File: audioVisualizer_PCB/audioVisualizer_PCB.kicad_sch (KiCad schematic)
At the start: 33 parts, among them J1 USB_C_Receptacle_USB2.0_16P, J3 SPI_LED_MATRIX, U2 HT7333, U7 STM32F401CCUx, Y1 ASE-25MHz

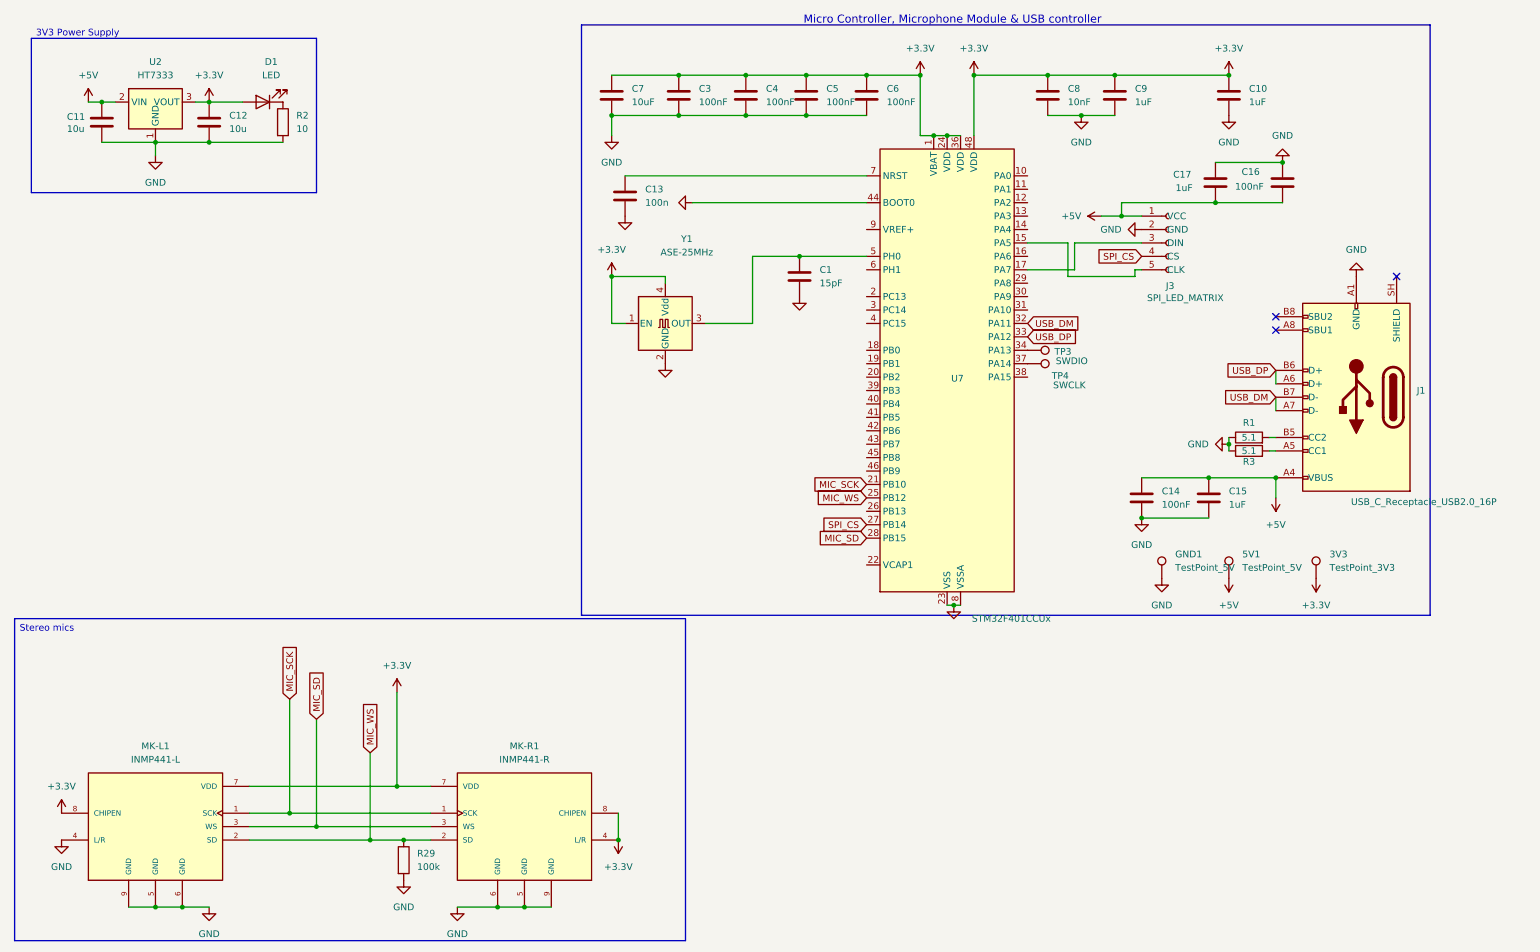
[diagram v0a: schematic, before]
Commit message: update
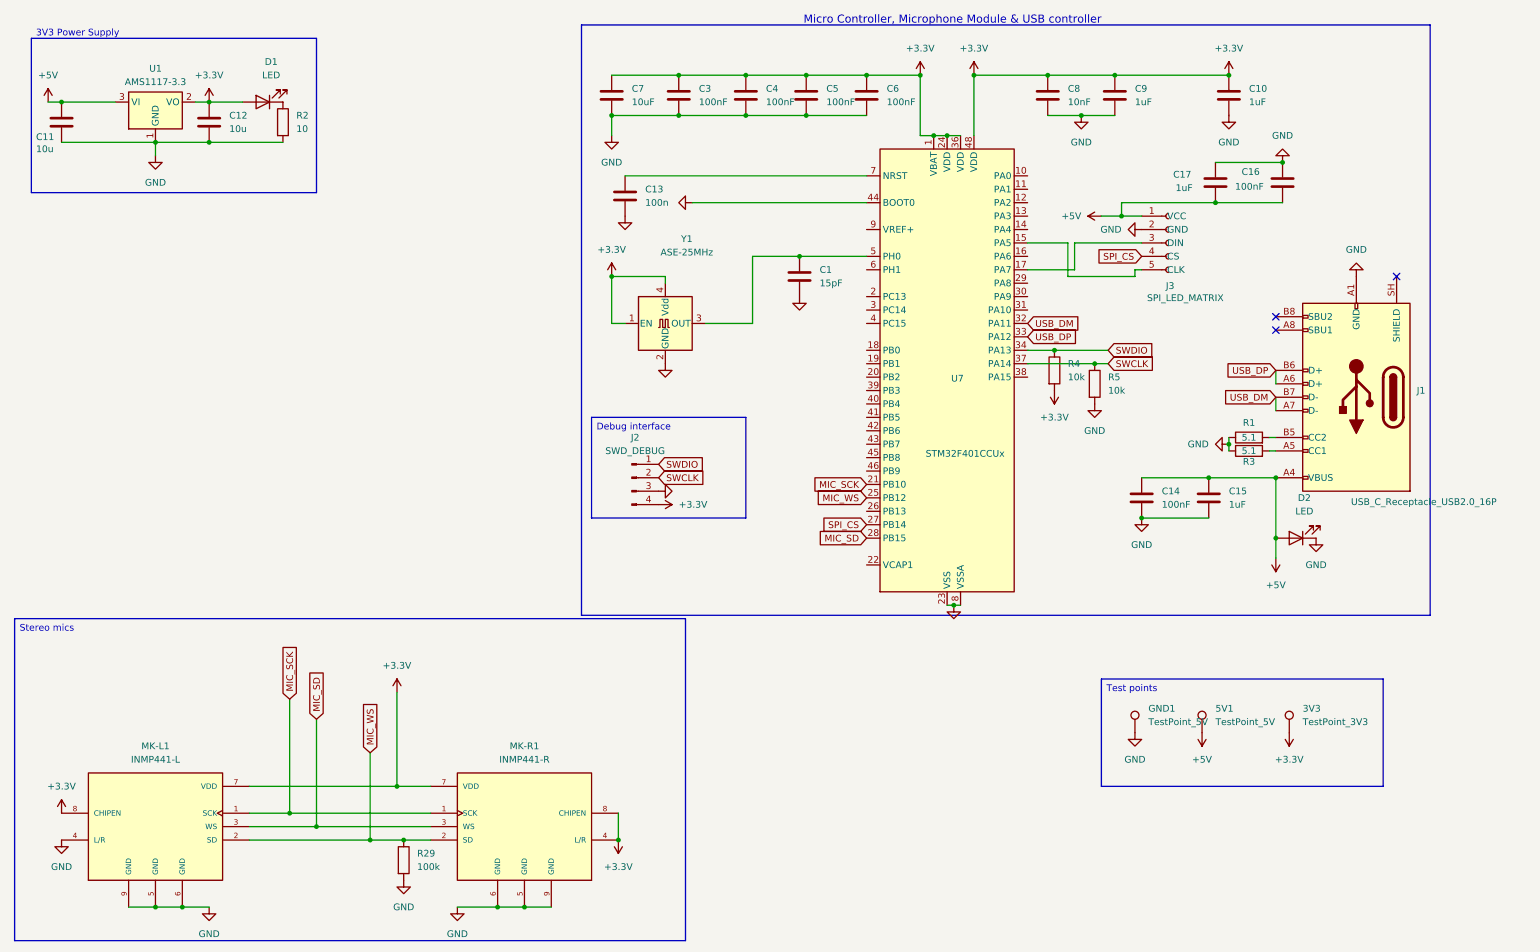
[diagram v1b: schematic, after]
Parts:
- removed TP3: SWDIO, TestPoint:TestPoint_Pad_1.0x1.0mm, symbol Connector:TestPoint
- removed TP4: SWCLK, TestPoint:TestPoint_Pad_1.0x1.0mm, symbol Connector:TestPoint
- removed U2: HT7333, Package_TO_SOT_SMD:SOT-89-3, symbol Regulator_Linear:HT75xx-1-SOT89
- added D2: LED, LED_SMD:LED_0805_2012Metric, symbol Device:LED
- added J2: SWD_DEBUG, Connector_PinHeader_2.54mm:PinHeader_1x04_P2.54mm_Vertical, symbol Connector:Conn_01x04_Pin
- added R4, R5: 10k, symbol Device:R
- added U1: AMS1117-3.3, Package_TO_SOT_SMD:SOT-223-3_TabPin2, symbol Regulator_Linear:AMS1117-3.3
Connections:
- net +3.3V: now also J2.4 (Pin_4), R4.2, U1.2 (VO)
- net +5V: now also D2.2 (A), U1.3 (VI)
- net GND: now also D2.1 (K), J2.3 (Pin_3), R5.2, U1.1 (GND)
- net SWDIO: now reaches U7.34 (PA13)
- net SWDIO: now also J2.1 (Pin_1), R4.1
- net SWCLK: now reaches U7.37 (PA14)
- net SWCLK: now also J2.2 (Pin_2), R5.1
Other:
- moved on the sheet: 3V3, 5V1, C11, GND1

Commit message: update
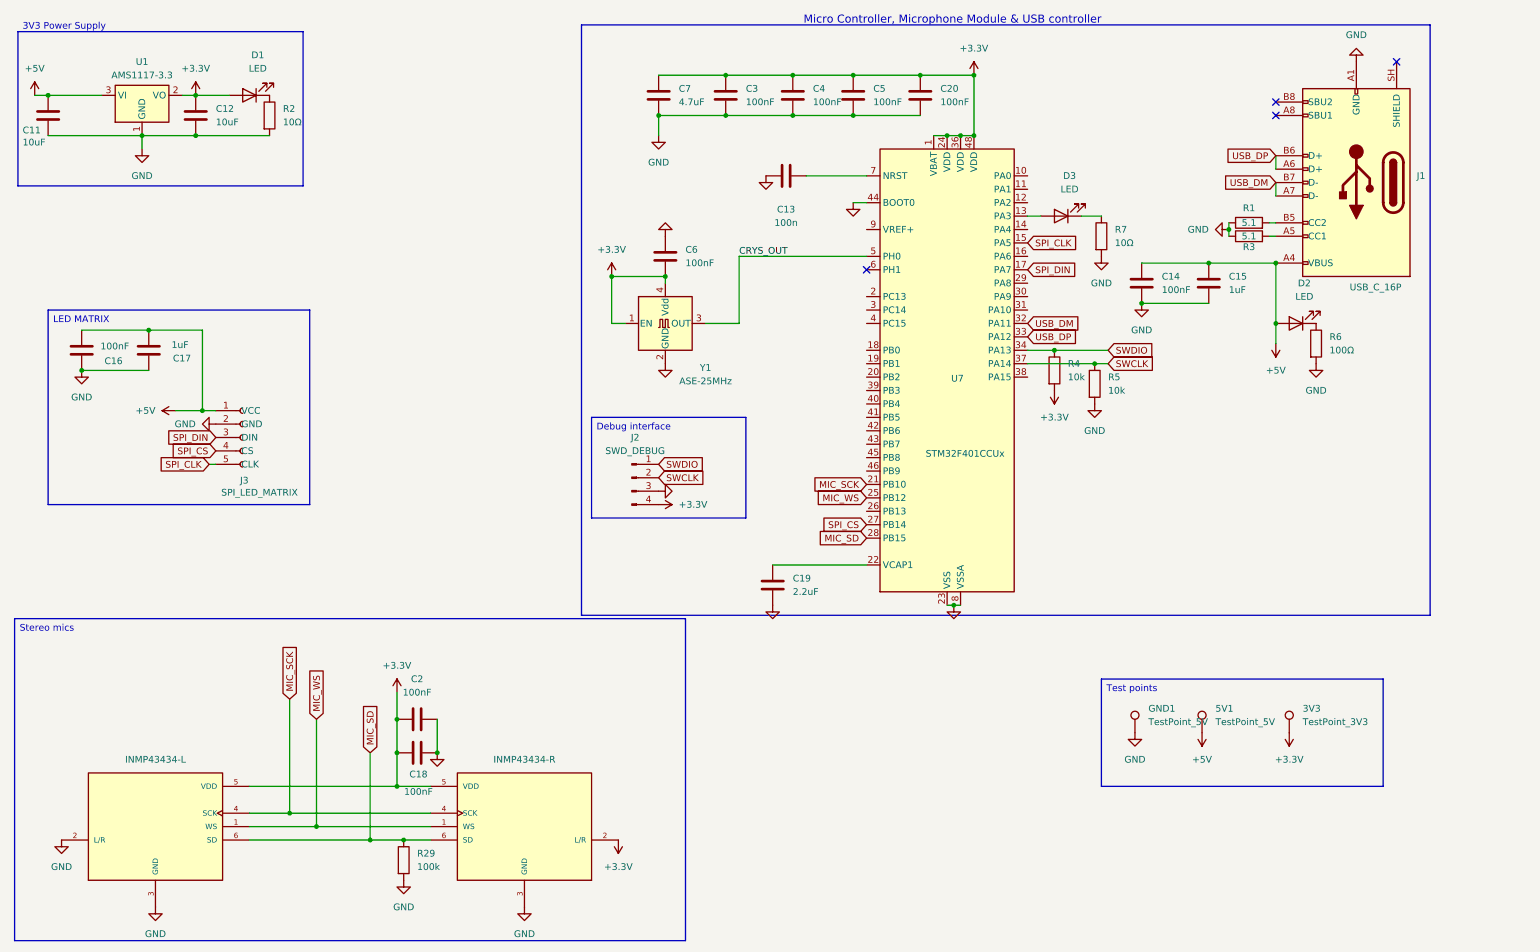
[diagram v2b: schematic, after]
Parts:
- removed C1: 15pF, Capacitor_SMD:C_0805_2012Metric, symbol Device:C
- removed C10, C9: 1uF, Capacitor_SMD:C_0805_2012Metric, symbol Device:C
- removed C8: 10nF, Capacitor_SMD:C_0805_2012Metric, symbol Device:C
- added C18, C2, C20: 100nF, Capacitor_SMD:C_0805_2012Metric, symbol Device:C
- added C19: 2.2uF, Capacitor_SMD:C_0805_2012Metric, symbol Device:C
- added D3: LED, LED_SMD:LED_0805_2012Metric, symbol Device:LED
- added R6: 100Ω, Resistor_SMD:R_0805_2012Metric, symbol Device:R
- added R7: 10Ω, Resistor_SMD:R_0805_2012Metric, symbol Device:R
- C11, C12: value 10u -> 10uF
- C7: value 10uF -> 4.7uF
- J1: value USB_C_Receptacle_USB2.0_16P -> USB_C_16P
- MK-L1: value INMP441-L -> INMP43434-L; footprint Custom:MIC_INMP441ACEZ-R7 -> Custom:MIC_ICS-43434
- MK-R1: value INMP441-R -> INMP43434-R; footprint Custom:MIC_INMP441ACEZ-R7 -> Custom:MIC_ICS-43434
- R2: value 10 -> 10Ω
- R4, R5: footprint (none) -> Resistor_SMD:R_0805_2012Metric
- Y1: footprint Oscillator:Oscillator_SMD_Abracon_ASE-4Pin_3.2x2.5mm -> Oscillator:Oscillator_SMD_EuroQuartz_XO32-4Pin_3.2x2.5mm
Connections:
- net +3.3V: now also C6.2, MK-L1.5 (VDD), MK-R1.2 (L/R), MK-R1.5 (VDD), C18.2, C2.1, C20.1; no longer C6.1, MK-L1.7 (VDD), MK-L1.8 (CHIPEN), MK-R1.4 (L/R), MK-R1.7 (VDD), MK-R1.8 (CHIPEN)
- net GND: now also C6.1, MK-L1.2 (L/R), MK-L1.3 (GND), MK-R1.3 (GND), C18.1, C19.2, C2.2, C20.2, R6.2, R7.2; no longer C6.2, D2.1 (K), MK-L1.4 (L/R), MK-L1.5 (GND), MK-L1.6 (GND), MK-L1.9 (GND), MK-R1.5 (GND), MK-R1.6 (GND), MK-R1.9 (GND)
- net MIC_SCK: now also MK-L1.4 (SCK), MK-R1.4 (SCK); no longer MK-L1.1 (SCK), MK-R1.1 (SCK)
- net MIC_SD: now also MK-L1.6 (SD), MK-R1.6 (SD), R29.1; no longer MK-L1.3 (WS), MK-R1.3 (WS)
- net MIC_WS: now also MK-L1.1 (WS), MK-R1.1 (WS); no longer MK-L1.2 (SD), MK-R1.2 (SD), R29.1
- net at U7.13 (PA3): now also D3.2 (A)
- net SPI_CLK: now reaches J3.5 (CLK), U7.15 (PA5)
- net SPI_DIN: now reaches J3.3 (DIN), U7.17 (PA7)
- net at U7.22 (VCAP1): now also C19.1
- net CRYS_OUT: now reaches U7.5 (PH0), Y1.3 (OUT)
- new net: D2.1 (K), R6.1
- new net: D3.1 (K), R7.1
- no-connect marks 3 -> 4
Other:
- moved on the sheet: C11, C12, C13, C14, C15, C16, C17, C3, C4, C5, C7, D1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
